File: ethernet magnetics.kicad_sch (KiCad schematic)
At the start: 18 parts, among them T1 S558-5999-46-F

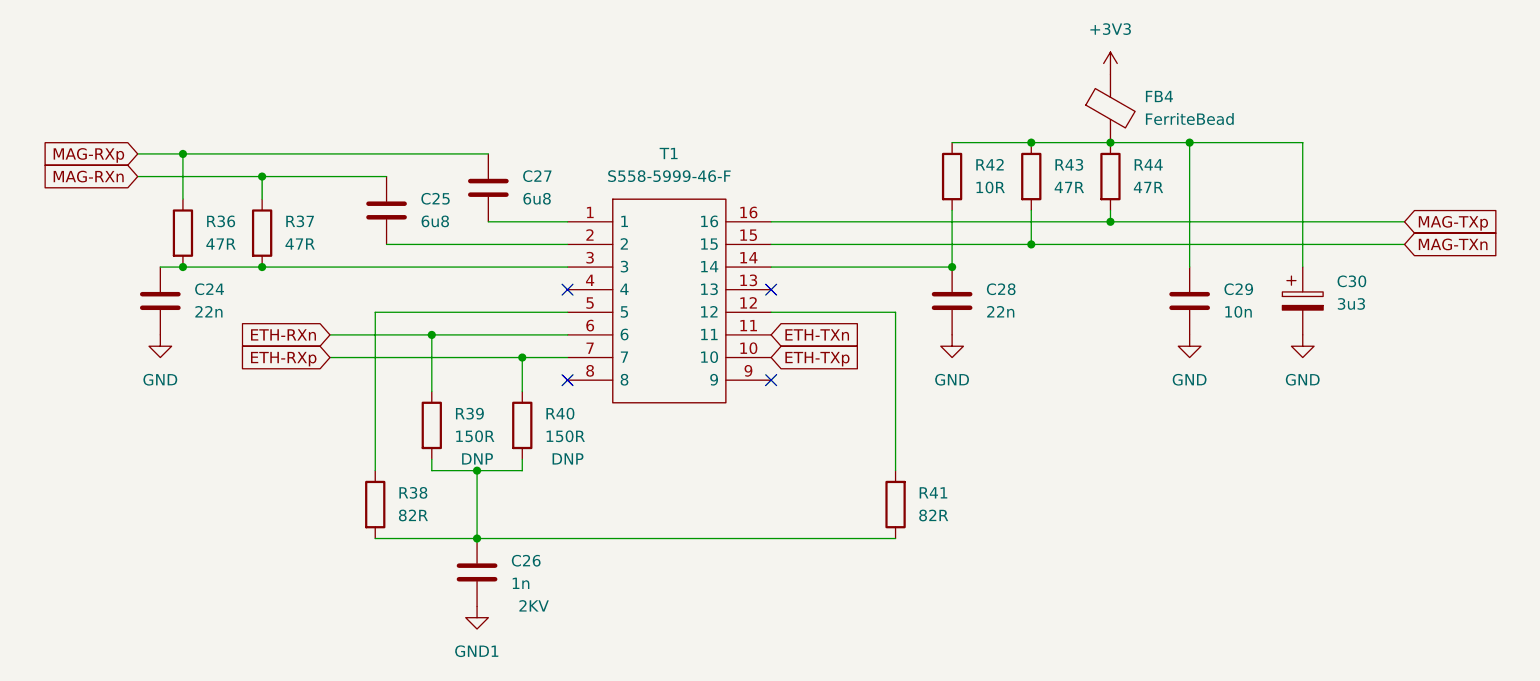
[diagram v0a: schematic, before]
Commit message: did a lot more routing, phy nearly done
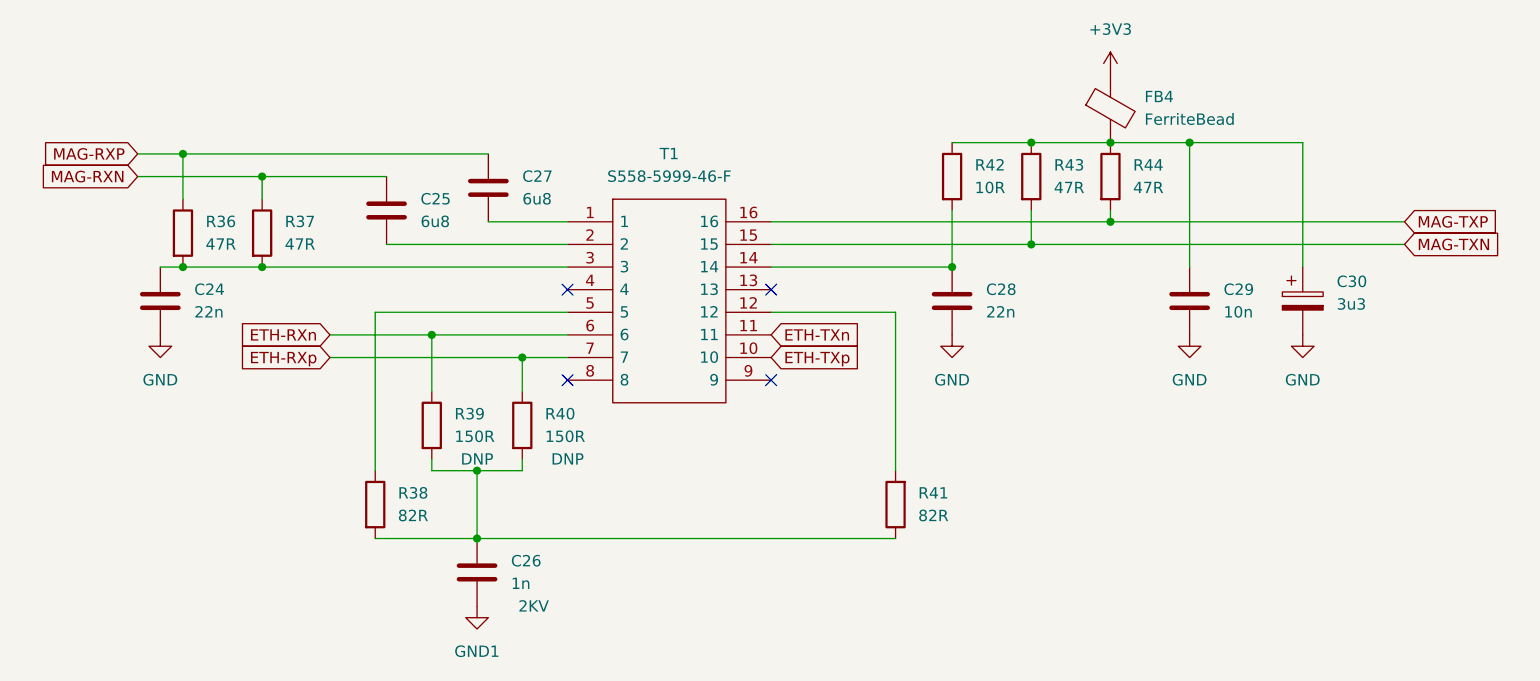
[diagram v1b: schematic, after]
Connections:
- net MAG-RXn renamed MAG-RXN
- net MAG-RXp renamed MAG-RXP
- net MAG-TXn renamed MAG-TXN
- net MAG-TXp renamed MAG-TXP
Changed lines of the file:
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@@
     (stroke (width 0) (type default) (color 0 0 0 0))
   )
-  (global_label "MAG-TXp" (shape input) (at 210.82 72.39 0) (fields_autoplaced)
+  (global_label "MAG-TXP" (shape input) (at 210.82 72.39 0) (fields_autoplaced)
     (effects (font (size 1.27 1.27)) (justify left))
-    (property "Intersheet References" "${INTERSHEET_REFS}" (id 0) (at 221.9417 72.4694 0)
+    (property "Intersheet References" "${INTERSHEET_REFS}" (id 0) (at 222.0626 72.3106 0)
       (effects (font (size 1.27 1.27)) (justify left) hide)
     )
   )
-  (global_label "MAG-RXp" (shape input) (at 68.58 64.77 180) (fields_autoplaced)
+  (global_label "MAG-RXP" (shape input) (at 68.58 64.77 180) (fields_autoplaced)
     (effects (font (size 1.27 1.27)) (justify right))
-    (property "Intersheet References" "${INTERSHEET_REFS}" (id 0) (at 57.1559 64.6906 0)
+    (property "Intersheet References" "${INTERSHEET_REFS}" (id 0) (at 57.035 64.6906 0)
       (effects (font (size 1.27 1.27)) (justify right) hide)
     )
@@
     )
   )
-  (global_label "MAG-RXn" (shape input) (at 68.58 67.31 180) (fields_autoplaced)
+  (global_label "MAG-RXN" (shape input) (at 68.58 67.31 180) (fields_autoplaced)
     (effects (font (size 1.27 1.27)) (justify right))
-    (property "Intersheet References" "${INTERSHEET_REFS}" (id 0) (at 57.1559 67.2306 0)
+    (property "Intersheet References" "${INTERSHEET_REFS}" (id 0) (at 56.9745 67.2306 0)
       (effects (font (size 1.27 1.27)) (justify right) hide)
     )
@@
     )
   )
-  (global_label "MAG-TXn" (shape input) (at 210.82 74.93 0) (fields_autoplaced)
+  (global_label "MAG-TXN" (shape input) (at 210.82 74.93 0) (fields_autoplaced)
     (effects (font (size 1.27 1.27)) (justify left))
-    (property "Intersheet References" "${INTERSHEET_REFS}" (id 0) (at 221.9417 75.0094 0)
+    (property "Intersheet References" "${INTERSHEET_REFS}" (id 0) (at 222.1231 74.8506 0)
       (effects (font (size 1.27 1.27)) (justify left) hide)
     )
